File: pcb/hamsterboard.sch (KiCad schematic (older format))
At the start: 2 parts

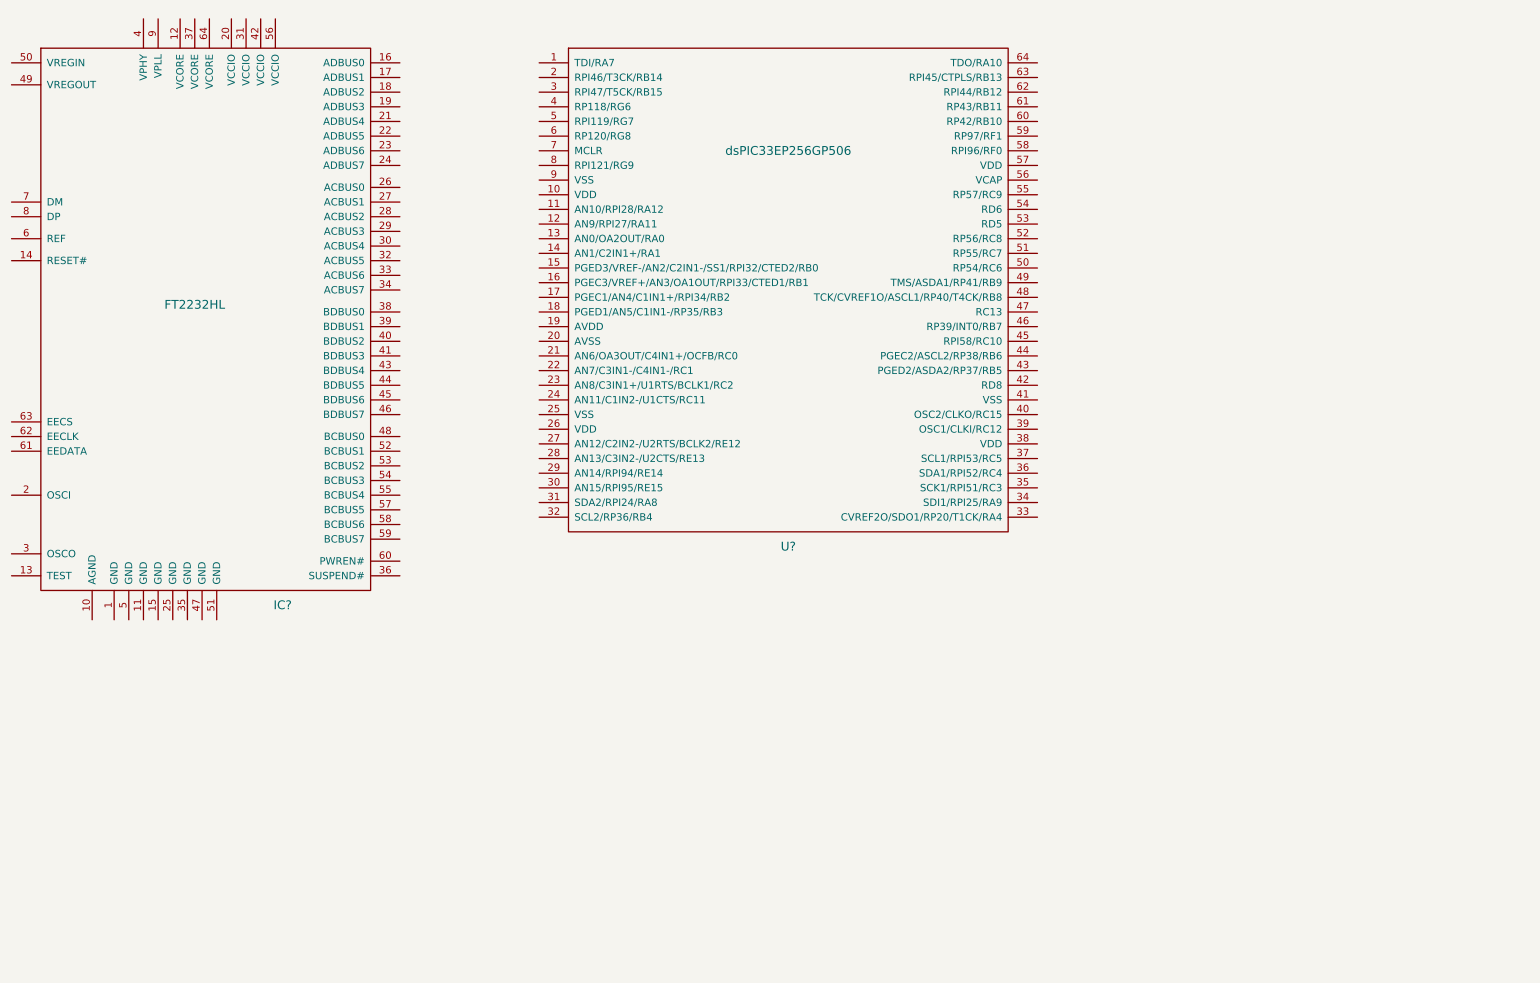
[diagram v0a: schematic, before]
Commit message: hamsterboard.sch
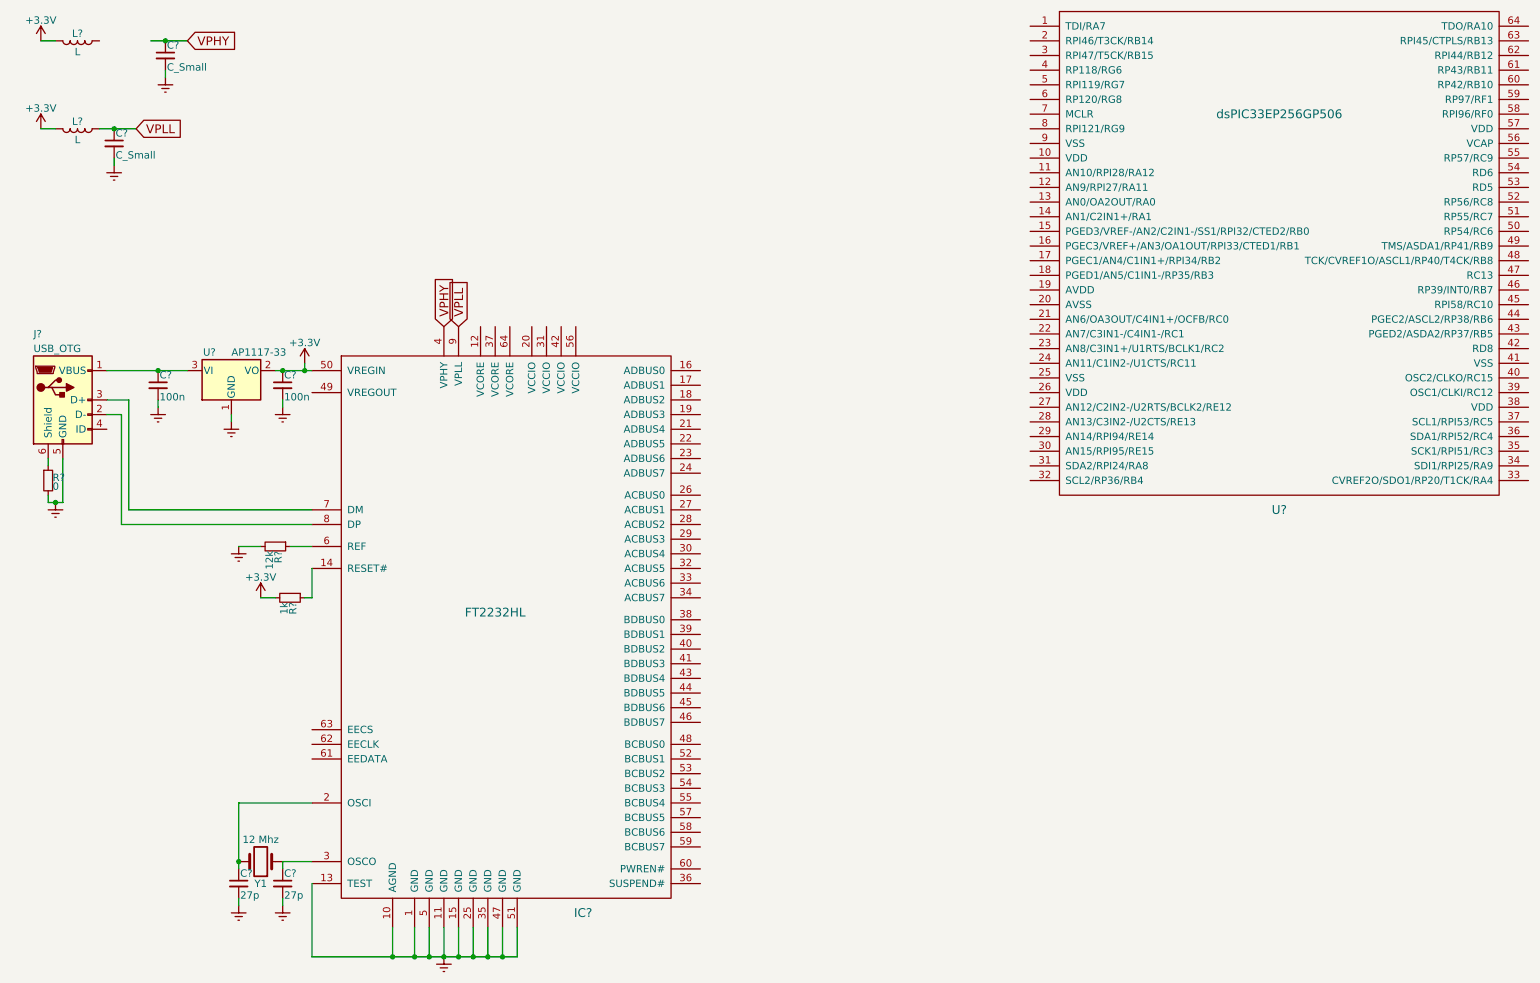
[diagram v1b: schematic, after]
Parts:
- added C? (x2): C_Small, symbol C_Small
- added C? (x2): 27p, symbol C_Small
- added C? (x2): 100n, symbol C_Small
- added J?: USB_OTG, symbol USB_OTG
- added L? (x2): L, symbol L
- added R?: 0, symbol R_Small
- added R?: 12k, symbol R_Small
- added R?: 1k, symbol R_Small
- added U?: AP1117-33, TO_SOT_Packages_SMD:SOT-223-3Lead_TabPin2, symbol AP1117-33
- added Y1: 12 Mhz, symbol Crystal
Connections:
- net Earth: now reaches IC?.1 (GND)
- net Earth: now also IC?.10 (AGND), IC?.11 (GND), IC?.13 (TEST), IC?.15 (GND), IC?.25 (GND), IC?.35 (GND), IC?.47 (GND), IC?.5 (GND), IC?.51 (GND), C?.2, C?.2, C?.2, C?.2, C?.2, C?.2, J?.5 (GND), R?.2, R?.2, U?.1 (GND)
- net at IC?.14 (RESET#): now also R?.1
- net at IC?.2 (OSCI): now also C?.1, Y1.2
- net at IC?.3 (OSCO): now also C?.1, Y1.1
- net VPHY: now reaches IC?.4 (VPHY)
- net VPHY: now also C?.1
- net +3V3: now reaches IC?.50 (VREGIN)
- net +3V3: now also C?.1, L?.2, L?.2, R?.2, U?.2 (VO)
- net at IC?.6 (REF): now also R?.1
- net at IC?.7 (DM): now also J?.3 (D+)
- net at IC?.8 (DP): now also J?.2 (D-)
- net VPLL: now reaches IC?.9 (VPLL)
- net VPLL: now also C?.1, L?.1
- new net: C?.1, J?.1 (VBUS), U?.3 (VI)
- new net: J?.6 (Shield), R?.1
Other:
- moved on the sheet: IC?, U?
